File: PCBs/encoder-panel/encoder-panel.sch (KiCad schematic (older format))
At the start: 42 parts, among them J1 Conn_01x05, U1 EN1AJ-B28

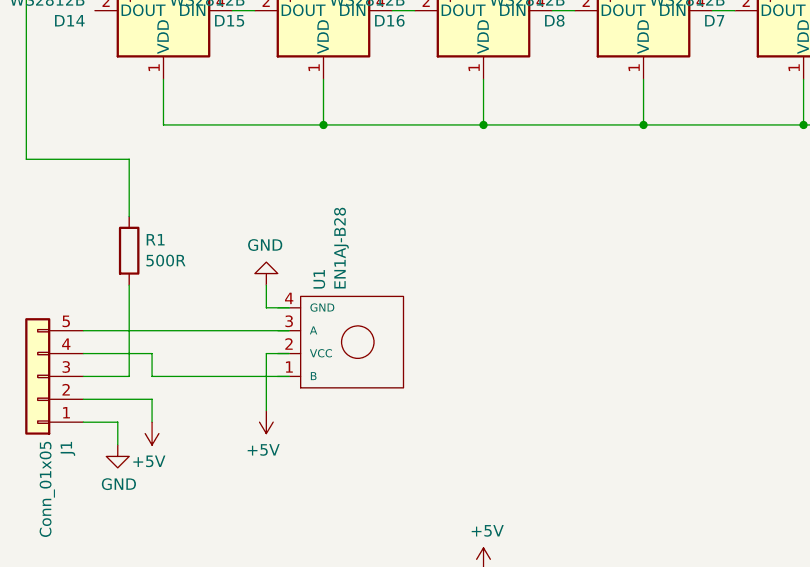
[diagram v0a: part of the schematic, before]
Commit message: misc fixes
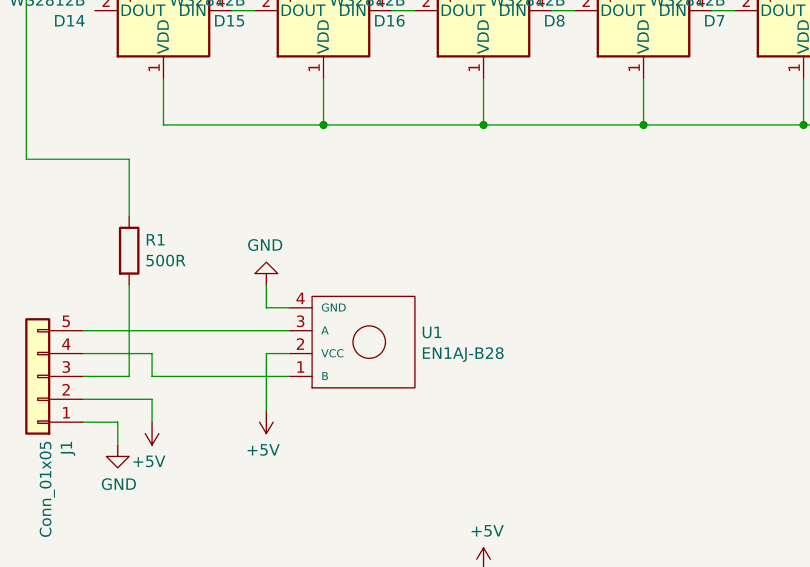
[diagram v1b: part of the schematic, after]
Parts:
- U1: footprint Bournes-EN:EN1AJ-B28-L100128L-H -> (none)
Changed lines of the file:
@@
-$EndComp
-$Comp
-L Bournes-EN-encoder:EN1AJ-B28 U1
-U 1 1 5BB4E9FF
-P 2500 3800
-F 0 "U1" H 2728 3967 50  0000 L CNN
-F 1 "EN1AJ-B28" H 2728 3876 50  0000 L CNN
-F 2 "Bournes-EN:EN1AJ-B28-L100128L-H" H 2500 3800 50  0001 C CNN
-F 3 "" H 2500 3800 50  0001 C CNN
-	1    2500 3800
-	0    -1   -1   0
 $EndComp
 $Comp
@@
 	1500 3550 1500 3950
 $Comp
-L power:GND #PWR?
+L power:GND #PWR0101
 U 1 1 5C535563
 P 2100 3550
-F 0 "#PWR?" H 2100 3300 50  0001 C CNN
+F 0 "#PWR0101" H 2100 3300 50  0001 C CNN
 F 1 "GND" H 2105 3377 50  0000 C CNN
 F 2 "" H 2100 3550 50  0001 C CNN
@@
 $EndComp
 $Comp
-L power:+5V #PWR?
+L power:+5V #PWR0102
 U 1 1 5C5355C2
 P 2100 4100
-F 0 "#PWR?" H 2100 3950 50  0001 C CNN
+F 0 "#PWR0102" H 2100 3950 50  0001 C CNN
 F 1 "+5V" H 2115 4273 50  0000 C CNN
 F 2 "" H 2100 4100 50  0001 C CNN
@@
 Wire Wire Line
 	2100 3650 2100 3550
+$Comp
+L Bournes-EN-encoder:EN1AJ-B28 U1
+U 1 1 5C55CD50
+P 2550 3800
+F 0 "U1" V 2591 3572 50  0000 R CNN
+F 1 "EN1AJ-B28" V 2500 3572 50  0000 R CNN
+F 2 "" H 2550 3850 50  0001 C CNN
+F 3 "" H 2550 3850 50  0001 C CNN
+	1    2550 3800
+	0    -1   -1   0
+$EndComp
 $EndSCHEMATC
